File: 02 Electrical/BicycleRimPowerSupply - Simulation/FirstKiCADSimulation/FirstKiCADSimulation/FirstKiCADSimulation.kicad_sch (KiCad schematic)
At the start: 8 parts

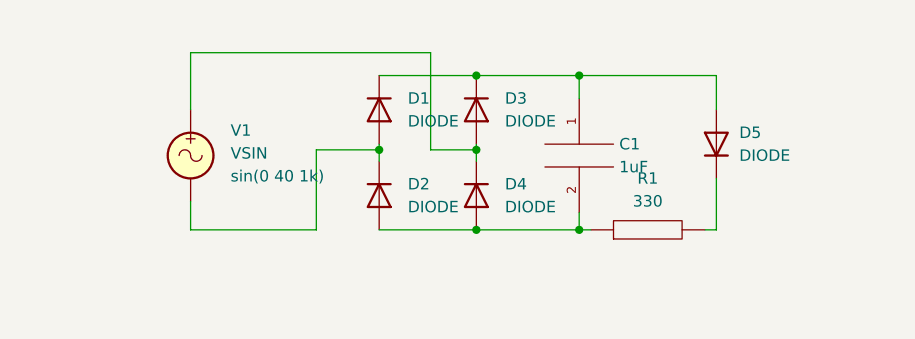
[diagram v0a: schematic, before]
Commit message: Experiments with simulations
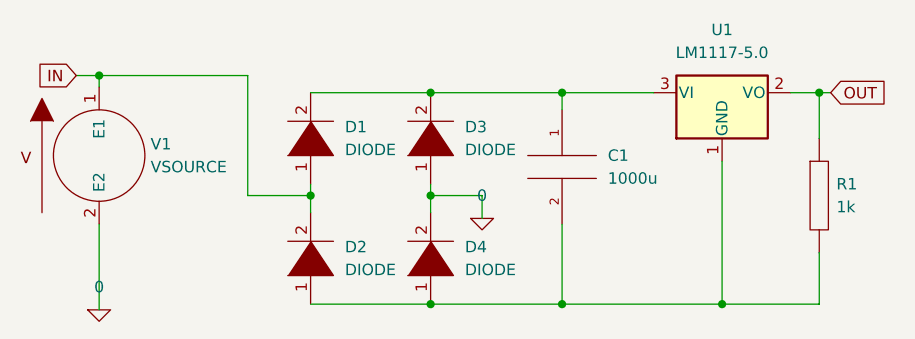
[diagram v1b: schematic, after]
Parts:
- removed D1, D2, D3, D4, D5: DIODE, symbol Simulation_SPICE:DIODE
- removed V1: VSIN, symbol Simulation_SPICE:VSIN
- added D1, D2, D3, D4: DIODE, symbol pspice:DIODE
- added U1: LM1117-5.0, symbol Regulator_Linear:LM1117-5.0
- added V1: VSOURCE, symbol pspice:VSOURCE
- C1: value 1uF -> 1000u; Spice_Model (none) -> 1000u; Spice_Netlist_Enabled (none) -> Y; Spice_Primitive (none) -> C
- R1: value 330 -> 1k; Spice_Model (none) -> 300; Spice_Netlist_Enabled (none) -> Y; Spice_Primitive (none) -> R
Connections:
- net at C1.1: now also D1.2 (A), D3.2 (A), U1.3 (VI)
- net at R1.2: now also C1.2, D2.1 (K), D4.1 (K), U1.1 (GND)
- net OUT: now reaches R1.1
- net OUT: now also U1.2 (VO); no longer C1.2
- new net 0: D3.1 (K), D4.2 (A), V1.2 (E2)
- new net IN: D1.1 (K), D2.2 (A), V1.1 (E1)
